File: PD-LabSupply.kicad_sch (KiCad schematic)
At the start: 86 parts, among them J1 Conn_01x02, J3 USB_C_Receptacle_USB2.0, J6 Conn_01x07, J8 Conn_02x02_Counter_Clockwise, Q1 BC847, Q4 IRF9393, SW1 SW_DIP_x06, SW2 SW_DPST_x2, SW3 SW_Push, SW4 SW_Push, SW5 SW_DPST_x2, SW6 SW_Push, U1 SRV05-4, U3 TMCS1108, U4 AP33772, U5 RP2040, U6 oledSym, U7 LMR54410, U8 AP2112K-3.3TRG1, U9 W25Q16JVSSIQ, Y1 Crystal_GND24

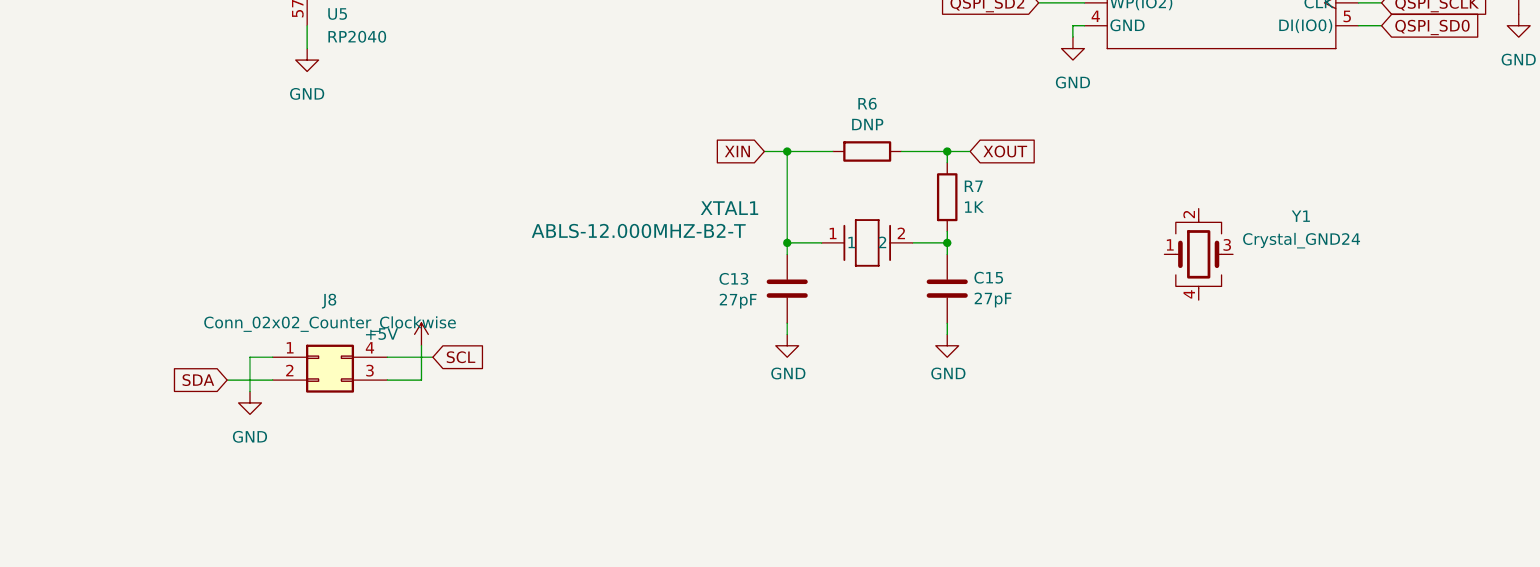
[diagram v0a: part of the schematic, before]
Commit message: save
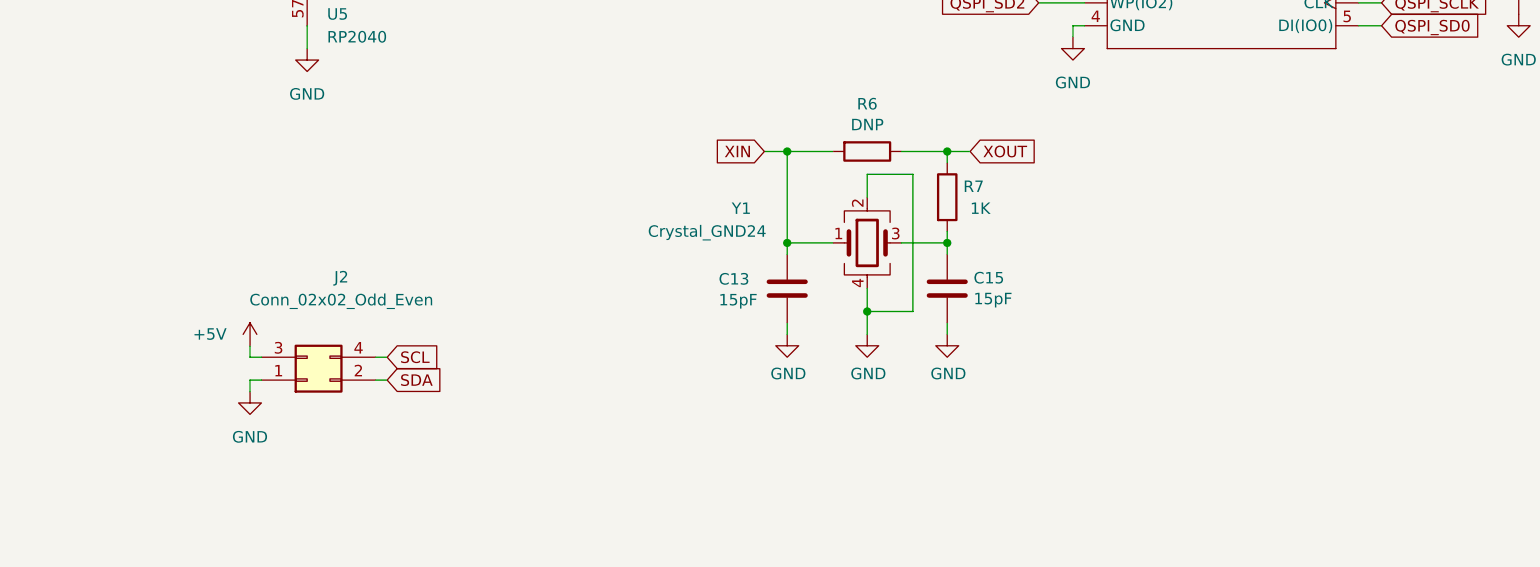
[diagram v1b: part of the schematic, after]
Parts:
- removed J8: Conn_02x02_Counter_Clockwise, Connector_PinSocket_2.54mm:PinSocket_2x02_P2.54mm_Horizontal, symbol Connector_Generic:Conn_02x02_Counter_Clockwise
- removed XTAL1: ABLS-12.000MHZ-B2-T, ABLS_12_000MHZ_B2_T:XTAL_HC&slash_49US_ABLS_ABR, symbol ABLS_12_000MHZ_B2_T:ABLS-12.000MHZ-B2-T
- added J2: Conn_02x02_Odd_Even, symbol Connector_Generic:Conn_02x02_Odd_Even
- C13, C15: value 27pF -> 15pF
- Y1: footprint (none) -> Crystal:Crystal_SMD_3225-4Pin_3.2x2.5mm
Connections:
- net +5V: now also J2.3 (Pin_3)
- net GND: now also Y1.2, Y1.4, J2.1 (Pin_1)
- net SCL: now also J2.4 (Pin_4)
- net SDA: now also J2.2 (Pin_2)
- net XIN: now also Y1.1
- net at C15.1, R7.2: now also Y1.3
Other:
- moved on the sheet: Y1
